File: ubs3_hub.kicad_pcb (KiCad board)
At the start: 6 copper layers, 50 x 50 mm, 68 parts, among them J1 USB_C_Receptacle, J2 USB_C_Receptacle, J3 USB3_A, J4 USB3_A, J5 USB3_A, U2 CH213K, U3 CH217K, U4 CH217K, U5 CH217K, U6 CH217K, Y1 X322524MOB4SI

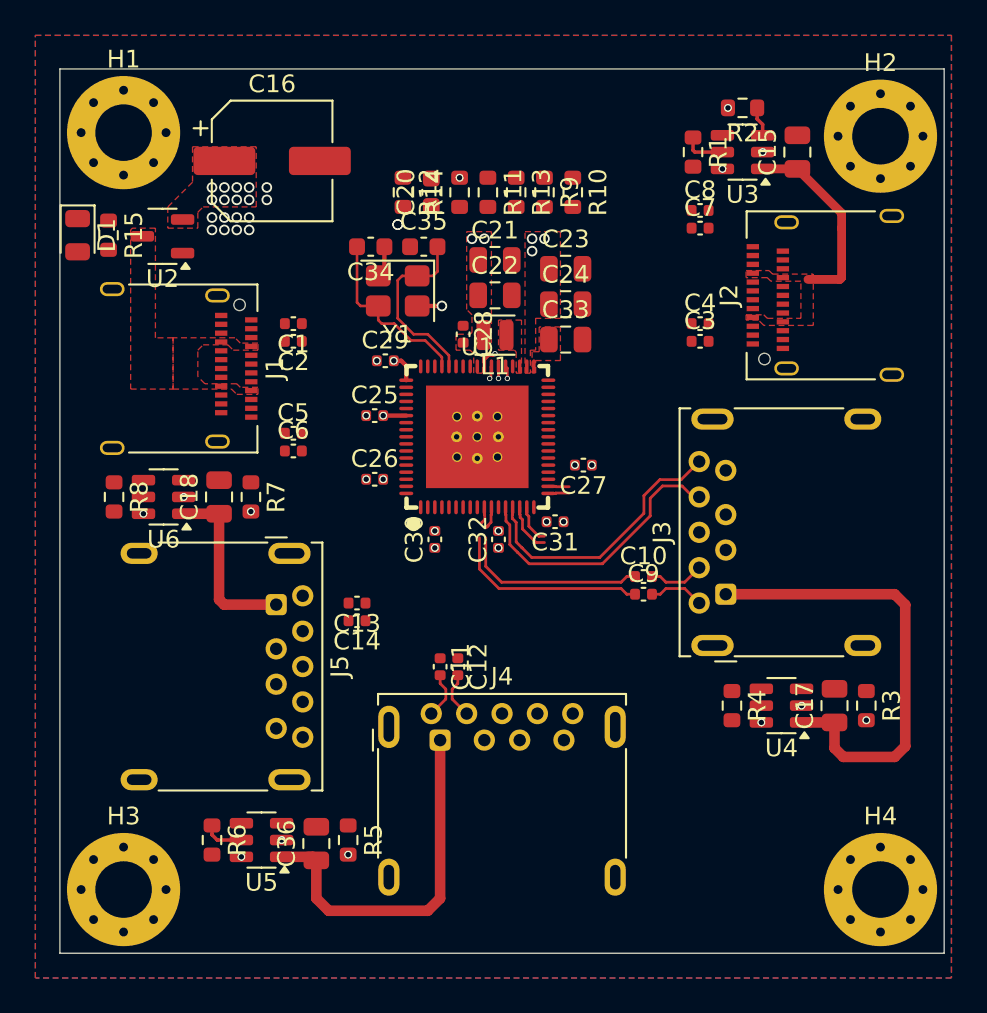
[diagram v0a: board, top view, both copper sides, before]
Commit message: Layout in progress
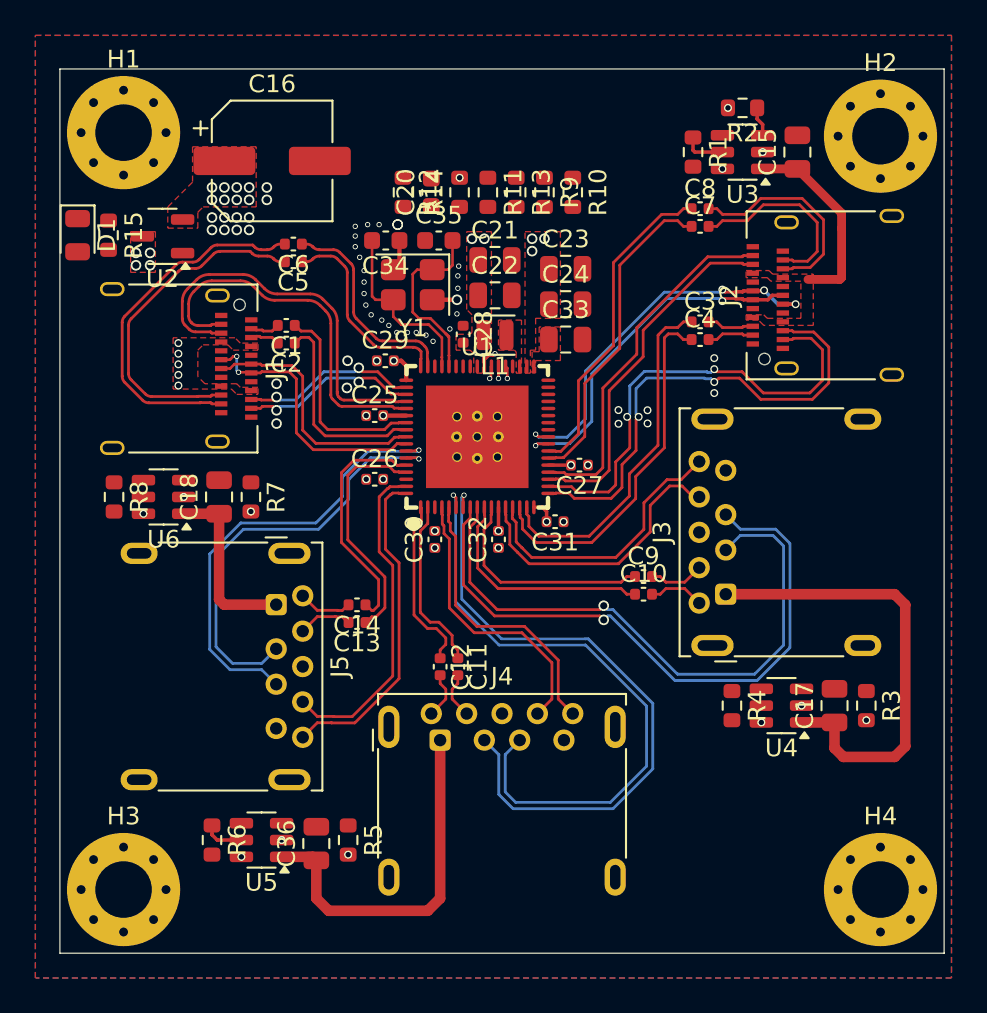
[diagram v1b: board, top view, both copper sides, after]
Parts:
- moved C6 11.7 mm to (85.0, 129.7), turned to 180 degrees
- moved C5 9.70 mm to (85.0, 130.7), turned to 180 degrees
- moved C13 1.10 mm to (88.6, 151.1)
- moved C3 1.10 mm to (108.0, 134.1)
- moved C10 1.00 mm to (104.8, 149.5)
- moved C11 1.00 mm to (94.3, 153.6)
- moved C12 1.00 mm to (93.3, 153.6)
- moved C9 1.00 mm to (104.8, 148.5)
- moved C34 0.92 mm to (90.2, 129.5)
- moved C35 0.92 mm to (93.2, 129.5)
- moved Y1 0.92 mm to (91.8, 132.0)
- moved C14 0.90 mm to (88.6, 150.1)
- moved C4 0.90 mm to (108.0, 135.1)
- moved C1 0.41 mm to (84.6, 134.3)
- moved C2 0.41 mm to (84.6, 135.3)
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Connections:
- C10 pad 1: /P2_SS_TXC_N -> /P2_SS_TXC_P
- C10 pad 2: /P2_SS_TX_N -> /P2_SS_TX_P
- C11 pad 1: /P3_SS_TXC_P -> /P3_SS_TXC_N
- C11 pad 2: /P3_SS_TX_P -> /P3_SS_TX_N
- C12 pad 1: /P3_SS_TXC_N -> /P3_SS_TXC_P
- C12 pad 2: /P3_SS_TX_N -> /P3_SS_TX_P
- C13 pad 1: /P4_SS_TXC_P -> /P4_SS_TXC_N
- C13 pad 2: /P4_SS_TX_P -> /P4_SS_TX_N
- C14 pad 1: /P4_SS_TXC_N -> /P4_SS_TXC_P
- C14 pad 2: /P4_SS_TX_N -> /P4_SS_TX_P
- C3 pad 1: /P1_SS_TXC_P -> /P1_SS_TXC_N
- C3 pad 2: /P1_SS_TX_P -> /P1_SS_TX_N
- C4 pad 1: /P1_SS_TXC_N -> /P1_SS_TXC_P
- C4 pad 2: /P1_SS_TX_N -> /P1_SS_TX_P
- C5 pad 1: /UPC_SS_TXC_P -> /UPC_SS_TXC_N
- C5 pad 2: /UPC_SS_TX_P -> /UPC_SS_TX_N
- C6 pad 1: /UPC_SS_TXC_N -> /UPC_SS_TXC_P
- C6 pad 2: /UPC_SS_TX_N -> /UPC_SS_TX_P
- C9 pad 1: /P2_SS_TXC_P -> /P2_SS_TXC_N
- C9 pad 2: /P2_SS_TX_P -> /P2_SS_TX_N
- U1 pad 1: /P3_SS_TXC_N -> /P3_SS_TXC_P
- U1 pad 10: /P2_SS_TXC_N -> /P2_SS_TXC_P
- U1 pad 11: /P2_SS_TXC_P -> /P2_SS_TXC_N
- U1 pad 15: /P1_SS_TXC_N -> /P1_SS_TXC_P
- U1 pad 16: /P1_SS_TXC_P -> /P1_SS_TXC_N
- U1 pad 2: /P3_SS_TXC_P -> /P3_SS_TXC_N
- U1 pad 20: /P1C_SS_RX_P -> /P1C_SS_RX_N
- U1 pad 21: /P1C_SS_RX_N -> /P1C_SS_RX_P
- U1 pad 4: /P3_SS_RX_N -> /P3_SS_RX_P
- U1 pad 5: /P3_SS_RX_P -> /P3_SS_RX_N
- U1 pad 50: /UPC_SS_TXC_N -> /UPC_SS_TXC_P
- U1 pad 51: /UPC_SS_TXC_P -> /UPC_SS_TXC_N
- U1 pad 55: /UP_SS_RX_P -> /UP_SS_RX_N
- U1 pad 56: /UP_SS_RX_N -> /UP_SS_RX_P
- U1 pad 64: /P4_SS_TXC_N -> /P4_SS_TXC_P
- U1 pad 65: /P4_SS_TXC_P -> /P4_SS_TXC_N
- U1 pad 67: /P4_SS_RX_N -> /P4_SS_RX_P
- U1 pad 68: /P4_SS_RX_P -> /P4_SS_RX_N
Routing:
- net /P3_HS_N: track 0.00 -> 37.0 mm, vias 0 -> 1
- net /P2_HS_P: track 0.00 -> 36.4 mm, vias 0 -> 1
- net /P3_HS_P: track 0.00 -> 35.8 mm, vias 0 -> 1
- net /P2_HS_N: track 0.00 -> 34.6 mm, vias 0 -> 1
- net /P1_SS_RX_N: track 1.19 -> 27.8 mm, vias 0 -> 2
- net /P1_SS_RX_P: track 1.19 -> 26.8 mm, vias 0 -> 2
- net /P4_HS_P: track 0.00 -> 25.6 mm, vias 0 -> 1
- net /P4_HS_N: track 0.00 -> 24.4 mm, vias 0 -> 1
- net /UP_SS_RX_N: track 0.00 -> 22.5 mm
- net /P1_HS_N: track 0.00 -> 21.7 mm, vias 0 -> 4
- net /UP_SS_RX_P: track 0.00 -> 21.3 mm
- net /UPC_SS_TX_P: track 0.00 -> 20.6 mm
- net /P1C_SS_RX_P: track 0.00 -> 20.3 mm
- net /P1C_SS_RX_N: track 0.00 -> 20.3 mm
- net /P1_HS_P: track 0.00 -> 20.0 mm, vias 0 -> 2
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- added copper zone on In3.Cu, net VBUS
